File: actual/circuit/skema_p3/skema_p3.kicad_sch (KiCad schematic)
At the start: 0 parts

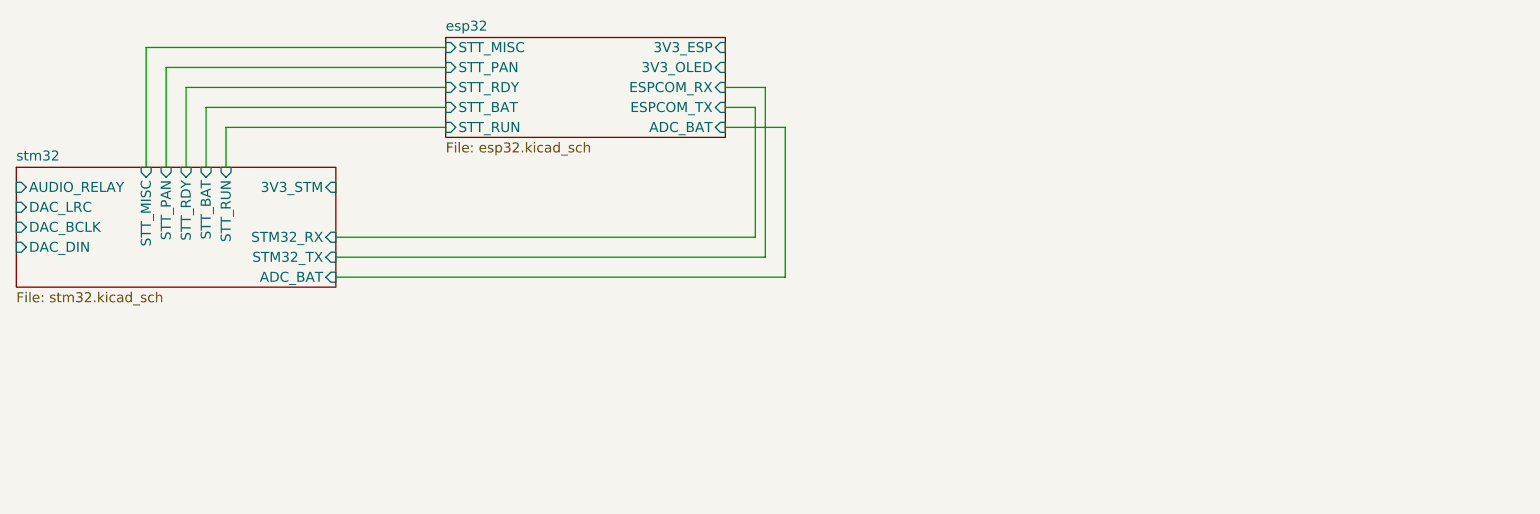
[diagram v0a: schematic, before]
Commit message: P3 in KiCAD
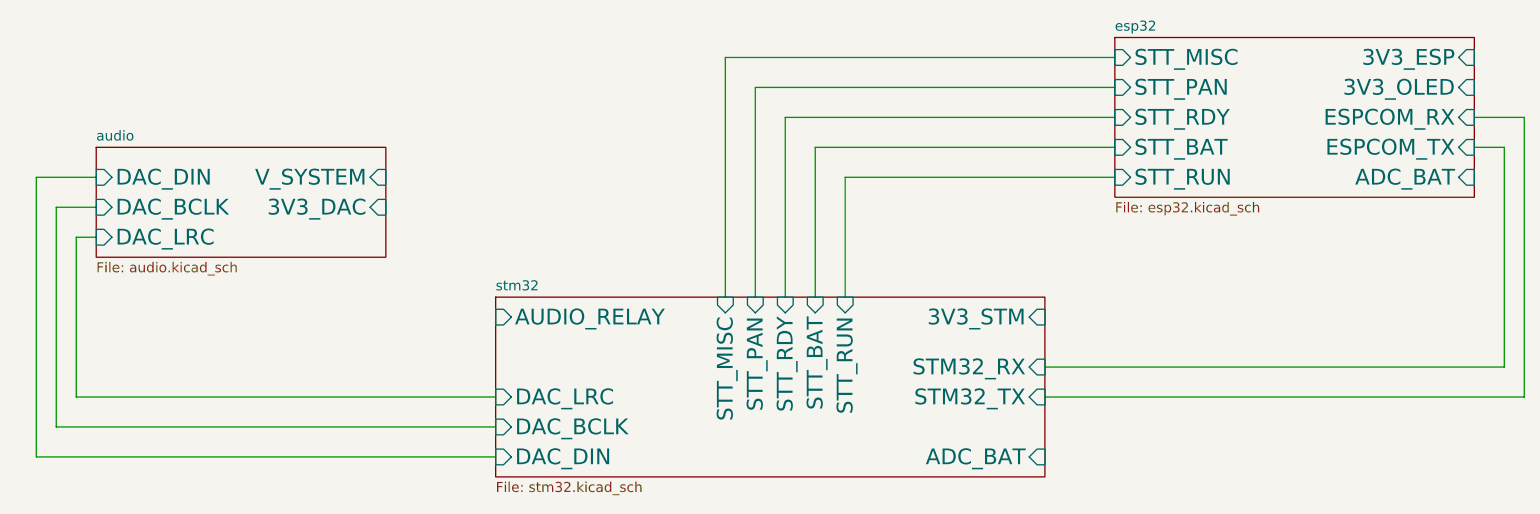
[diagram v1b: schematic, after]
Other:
- added sheet audio (audio.kicad_sch)
